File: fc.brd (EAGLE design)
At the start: 160 x 100 mm, 65 parts, among them IC1 FT230XQ, IC2 BN055, SW1 DHT-4235A, U2 ATMEGA2560-16AU100A-M, Y1 16MHz, Y2 32.768kHz

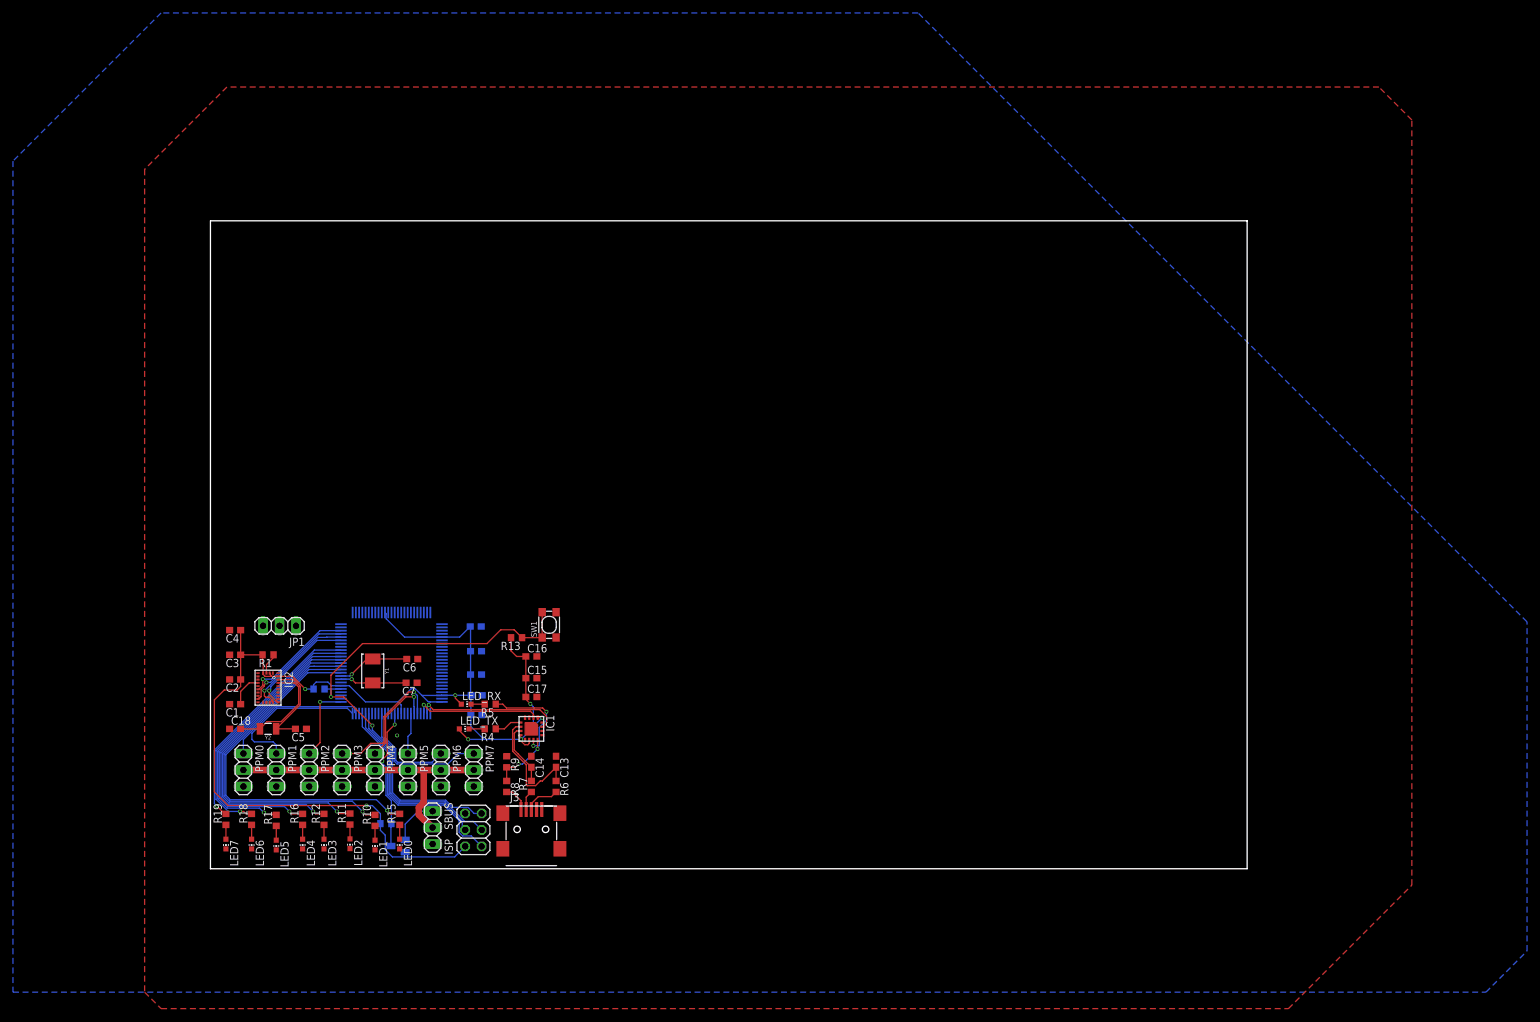
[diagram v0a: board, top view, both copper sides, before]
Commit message: Improved the design
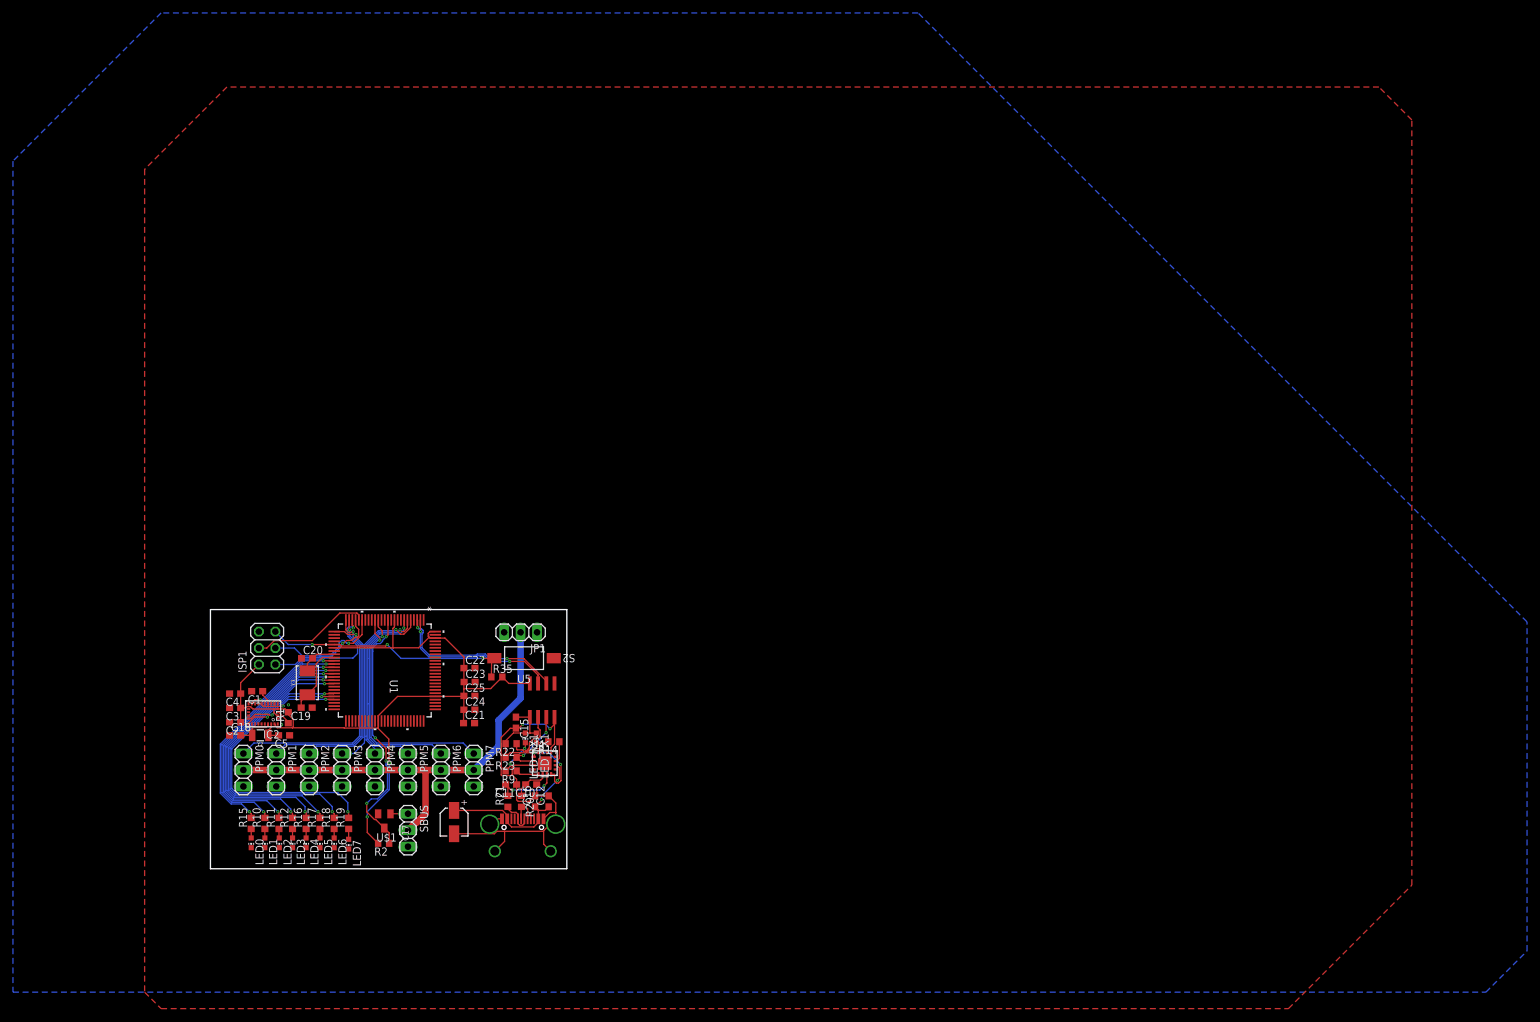
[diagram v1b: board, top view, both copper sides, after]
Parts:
- removed C13, C14: 47pF, rcl:C0603
- removed C6, C7: 8pF, rcl:C0603
- removed C8, C9: 100nF, rcl:C0603
- removed IC1: FT230XQ, ftdichip:QFN16
- removed ISP: (no value), pinhead:2X03
- removed J3: (no value), adafruit:USB-MINIB
- removed LED_RX, LED_TX: (no value), led:CHIP-LED0603
- removed R13: 10k, resistor:R0603
- removed R3: 10k, rcl:R0603
- removed R4, R5: 5.6, rcl:R0603
- removed R6, R7: 27, rcl:R0603
- removed R8: 4k7, rcl:R0603
- removed SW1: DHT-4235A, Seeed-Switch:SW4-SMD-4.2X3.2X2.5MM
- removed U2: ATMEGA2560-16AU100A-M, ATMEGA2560:100A-M
- removed Y1: 16MHz, SparkFun-Clocks:CRYSTAL-SMD-5X3.2-2PAD
- added C19, C20: 8pF, rcl:C0603
- added C21, C22, C23, C24, C25: 100nF, rcl:C0603
- added ISP1: (no value), pinhead:2X03
- added J2: USBC, USBC:USBC
- added LED_RX1, LED_TX1: (no value), led:CHIP-LED0603
- added R14: 270, rcl:R0603
- added R20, R21: 27, rcl:R0603
- added R22, R23: 4k7, rcl:R0603
- added R35: 10k, resistor:R0603
- added S2: FSMSM, switch:SWITCH_FSMSM
- added U1: ATMEGA2560-16AU100A-M, ATMEGA2560:100A-M
- added U4: FT230XQ, ftdichip:QFN16
- added U5: (no value), SI8621AB-B-IS:SO08
- added Y3: 16MHz, SparkFun-Clocks:CRYSTAL-SMD-5X3.2-2PAD
- C10, C11: value 100nF -> 47pF
- C12: value 100nF -> 10nF
- C17: device rcl:C0603 -> Kondensatoren (rev17a):2.6X1.6X1(BXCXA)
- R9: value 10k -> 270
- moved JP1 37.2 mm to (47.9, 36.5)
- moved C12 29.2 mm to (52.2, 10.4), flipped to the top, turned to 90 degrees
- moved R15 22.9 mm to (6.29, 7.00)
- moved LED0 22.9 mm to (6.29, 4.00)
- moved C17 22.7 mm to (37.6, 7.20), turned to 90 degrees
- moved C16 22.4 mm to (50.1, 10.4), turned to 90 degrees
- moved C11 21.3 mm to (46.4, 13.0), flipped to the top
- moved R19 19.0 mm to (21.3, 7.00)
- moved LED7 18.9 mm to (21.3, 3.80)
- moved R10 17.0 mm to (8.40, 7.00)
- moved LED1 17.0 mm to (8.40, 4.00)
- moved C10 13.7 mm to (49.5, 13.0), flipped to the top
- moved R18 12.8 mm to (19.1, 7.00)
- moved LED6 12.7 mm to (19.1, 4.00)
- moved R11 11.0 mm to (10.6, 7.00)
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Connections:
- removed net N$10: J3.D+, R6.2
- removed net N$11: J3.D-, R7.1
- removed net N$16: J3.VBUS, R8.2
- removed net N$6: IC1.5, R4.1
- removed net N$7: IC1.11, R5.1
- removed net N$8: LED_TX.C, R4.2
- removed net N$9: LED_RX.C, R5.2
- removed net VBUS_SENSE: IC1.12, R8.1, R9.2
- new net D+1: J2.A6, J2.B6, R20.2
- new net D-1: J2.A7, J2.B7, R21.1
- new net GNDIO: C10.1, C11.1, C12.2, C15.2, C16.2, C17.2, J2.A1, J2.A12, J2.S1, J2.S2, J2.S3, J2.S4, U4.13, U4.3, U5.4
- new net N$32: C19.2, U1.34, Y3.P$2
- new net N$33: C20.2, U1.33, Y3.P$1
- new net RXD: R23.1, U4.2, U5.3
- new net TXD: R22.1, U4.15, U5.2
- new net USBDM1: C11.2, R21.2, U4.7
- new net USBDP1: C10.2, R20.1, U4.6
- new net VBUS: C12.1, C16.1, C17.1, J2.A4, J2.A9, U4.10
- new net VCCIO: C15.1, LED_RX1.A, LED_TX1.A, R22.2, R23.2, U4.1, U4.16, U4.8, U5.1
- net !BNO_RST: now also U1.47; no longer U2.48
- net !RESET: now also ISP1.5, R35.1, S2.2, U1.30; no longer ISP.5, R13.1, R3.1, SW1.1, SW1.2, U2.30
- net !SBUS: now also U1.12; no longer U2.12
- net +3V3: now also C21.1, C22.1, C23.1, C24.1, C25.1, ISP1.2, R35.2, U1.10, U1.100, U1.31, U1.61, U1.80, U1.98, U5.8; no longer C10.1, C11.1, C12.1, C15.1, C16.1, C17.1, C8.1, C9.1, IC1.1, IC1.10, IC1.8, ISP.2, LED_RX.A, LED_TX.A, R13.2, R3.2, U2.10, U2.100, U2.31, U2.61, U2.80, U2.98
- net BNO_INT: now also U1.23; no longer U2.47
- net BNO_RX: now also U1.46; no longer U2.46
- net BNO_TX: now also U1.45; no longer U2.45
- net GND: now also C19.1, C20.1, C21.2, C22.2, C23.2, C24.2, C25.2, ISP1.6, S2.1, U1.11, U1.32, U1.62, U1.81, U1.99, U5.5; no longer C10.2, C11.2, C12.2, C13.1, C14.1, C15.2, C16.2, C17.2, C6.1, C7.1, C8.2, C9.2, IC1.13, IC1.3, ISP.6, J3.GND, R9.1, SW1.3, SW1.4, U2.11, U2.32, U2.62, U2.81, U2.99
- net LED0: now also U1.35; no longer U2.35
- net LED1: now also U1.36; no longer U2.36
- net LED2: now also U1.37; no longer U2.37
- net LED3: now also U1.38; no longer U2.38
- net LED4: now also U1.39; no longer U2.39
- net LED5: now also U1.40; no longer U2.40
- net LED6: now also U1.41; no longer U2.41
- net LED7: now also U1.42; no longer U2.42
- net MISO: now also ISP1.1, U1.22; no longer ISP.1, U2.22
- net MOSI: now also ISP1.4, U1.21; no longer ISP.4, U2.21
- net N$2: now also R14.1, U4.11; no longer C6.2, U2.34, Y1.P$2
- net N$3: now also LED_RX1.C, R9.2; no longer C7.2, U2.33, Y1.P$1
- net N$4: now also LED_TX1.C, R14.2; no longer C13.2, IC1.6, R6.1
- net N$5: now also R9.1, U4.5; no longer C14.2, IC1.7, R7.2
- net PPM0: now also U1.24; no longer U2.24
- net PPM1: now also U1.25; no longer U2.25
- net PPM2: now also U1.26; no longer U2.26
- net PPM3: now also U1.5; no longer U2.5
- net PPM4: now also U1.6; no longer U2.6
- net PPM5: now also U1.7; no longer U2.7
- net PPM6: now also U1.15; no longer U2.15
- net PPM7: now also U1.16; no longer U2.16
- net SCK: now also ISP1.3, U1.20; no longer ISP.3, U2.20
- net USB_RX: now also U1.2, U5.7; no longer IC1.15, U2.2
- net USB_TX: now also U1.3, U5.6; no longer IC1.2, U2.3
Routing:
- net GNDIO: track 0.00 -> 74.6 mm, vias 0 -> 2
- net +3V3: track 194.7 -> 125.3 mm, vias 7 -> 2
- net !RESET: track 82.0 -> 39.7 mm, vias 2 -> 3
- net VCCIO: track 0.00 -> 28.7 mm, vias 0 -> 2
- net VBUS: track 0.00 -> 27.7 mm, vias 0 -> 2
- net +5V: track 71.1 -> 95.8 mm
- net PPM5: track 6.36 -> 29.7 mm, vias 0 -> 1
- net LED0: track 57.3 -> 37.2 mm, vias 1 -> 2
- net !SBUS: track 21.8 -> 40.1 mm, vias 2 -> 4
- net PPM2: track 11.9 -> 29.2 mm
- net N$4: track 18.6 -> 1.91 mm
- net PPM6: track 15.6 -> 31.6 mm, vias 0 -> 1
- net LED1: track 54.4 -> 38.5 mm, vias 1 -> 2
- net N$7: track 15.8 -> 0.00 mm, vias 2 -> 0
- net MISO: track 33.0 -> 17.5 mm, vias 0 -> 1
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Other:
- board size 160 x 100 mm -> 55 x 40 mm
